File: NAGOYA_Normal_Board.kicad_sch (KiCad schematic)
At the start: 93 parts, among them CN1 value, CN10 value, CN11 value, CN12 value, CN13 value, CN14 RefereeSystem, CN15 micro_B, CN2 value, CN3 value, CN4 value, CN5 value, CN6 value, CN7 value, CN8 value, CN9 value, J1 debug, Q2 DDTC114EUA-7-F, U1 Teensy4.1, U2 TCAN1042HVDR, U3 TCAN1042HVDR, U4 TCAN1042HVDR, U5 FT234XD, U6 TLP172AM, U7 BNO055, U9 LXES11DAA2-137, Y2 32.768 k

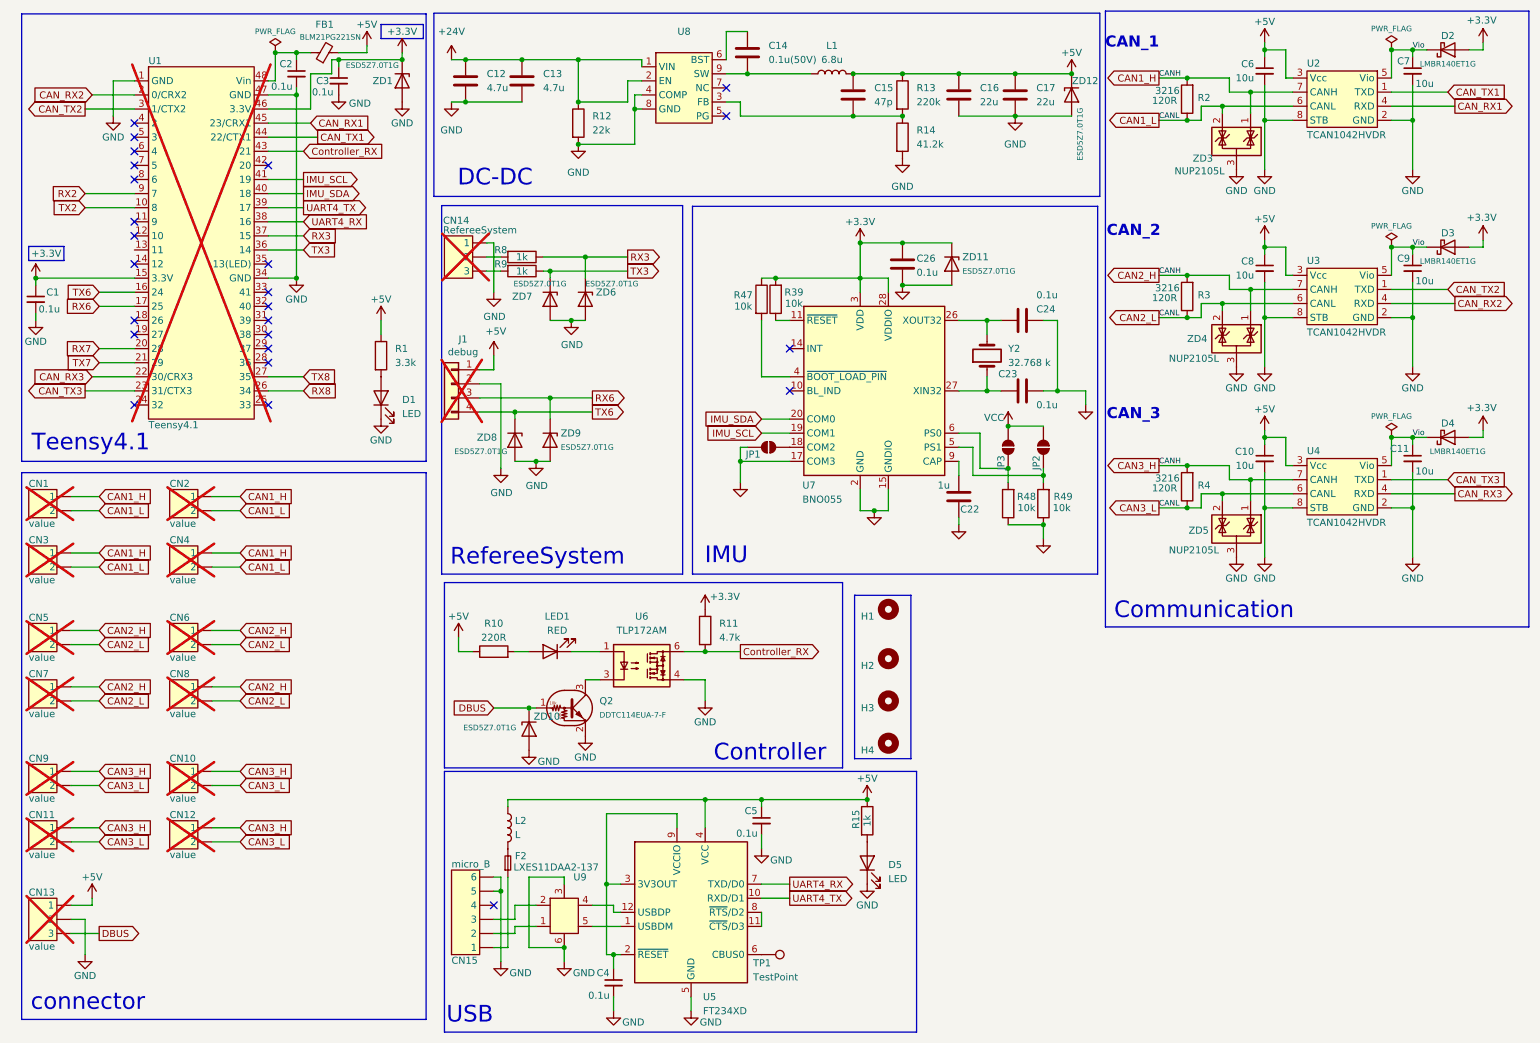
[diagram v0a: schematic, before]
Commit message: Update
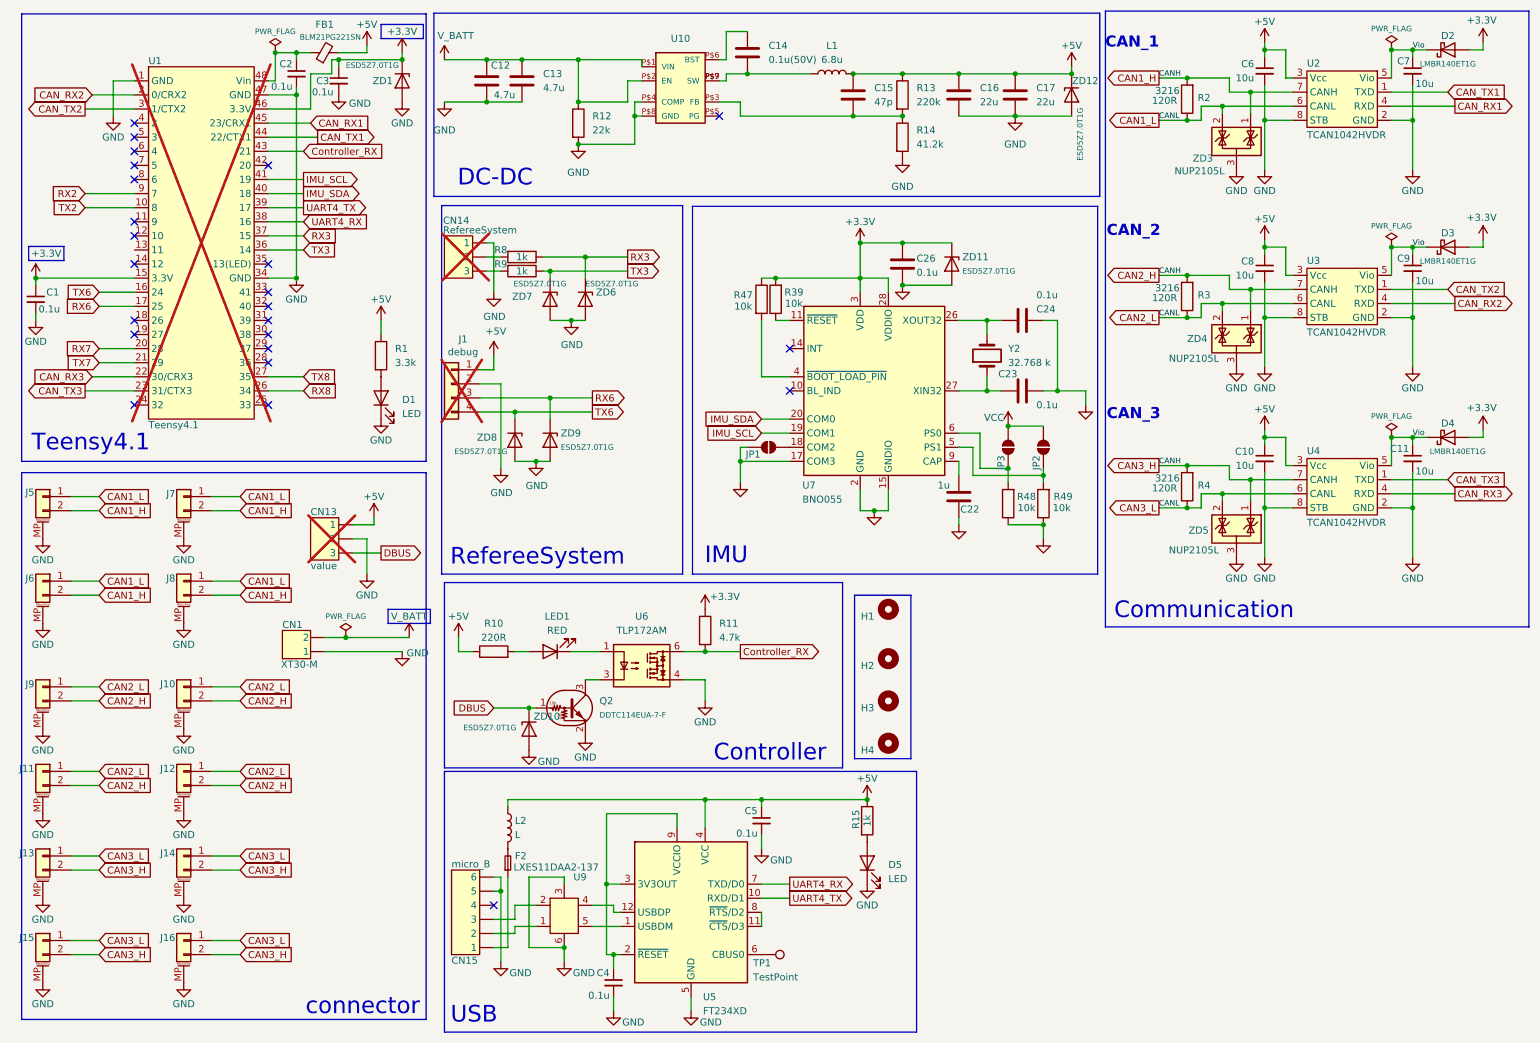
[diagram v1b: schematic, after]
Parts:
- removed CN10, CN11, CN12, CN2, CN3, CN4, CN5, CN6, CN7, CN8, CN9: value, symbol 0_circuit:CON_2P
- removed U8: ~, TanekonModule:V-DFN3020-13-A_L3.0-W2.0-P0.45-BL-EP_AP6335X, symbol TanekonModule:AP63357DV-7
- added J10, J11, J12, J13, J14, J15, J16, J5, J6, J7, J8, J9: CAN3, Connector_JST:JST_GH_SM02B-GHS-TB_1x02-1MP_P1.25mm_Horizontal, symbol Connector_Generic_MountingPin:Conn_01x02_MountingPin
- added U10: AP63357, 0_PCB:V-DFN3020-13, symbol AP63357:AP63357
- CN1: value value -> XT30-M; footprint (none) -> 0_PCB:AMASS_XT30PW-M_1x02_P2.50mm_Horizontal; LCSC (none) -> C428721; 型番 (none) -> XT30PW-M30.G.Y; 購入先 (none) -> JLCPCB; 購入先URL (none) -> https://jlcpcb.com/partdetail/Changzhou_AmassElec-XT30UM/C9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; now fitted
- CN13: footprint (none) -> Connector_PinHeader_2.54mm:PinHeader_1x03_P2.54mm_Vertical
- CN14: footprint (none) -> Connector_JST:JST_XH_B3B-XH-AM_1x03_P2.50mm_Vertical
- CN15: footprint (none) -> Connector_USB:USB_Micro-B_Amphenol_10118194-0001LF_Horizontal
- F2: footprint (none) -> Fuse:Fuse_0603_1608Metric; LCSC (none) -> C116602
- L2: footprint (none) -> Inductor_SMD:L_0603_1608Metric; LCSC (none) -> C85834
- U9: footprint (none) -> 0_PCB:FIL_LXES11DAA2-137
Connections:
- net CAN1_H: now also J10.2 (Pin_2), J11.2 (Pin_2), J12.2 (Pin_2), J13.2 (Pin_2), J14.2 (Pin_2), J15.2 (Pin_2), J16.2 (Pin_2), J5.2 (Pin_2), J6.2 (Pin_2), J7.2 (Pin_2), J8.2 (Pin_2), J9.2 (Pin_2); no longer CN1.1
- net CAN1_L: now also J10.1 (Pin_1), J11.1 (Pin_1), J12.1 (Pin_1), J13.1 (Pin_1), J14.1 (Pin_1), J15.1 (Pin_1), J16.1 (Pin_1), J5.1 (Pin_1), J6.1 (Pin_1), J7.1 (Pin_1), J8.1 (Pin_1), J9.1 (Pin_1); no longer CN1.2
- net GND: now also CN1.1, J10.MP (MountPin), J11.MP (MountPin), J12.MP (MountPin), J13.MP (MountPin), J14.MP (MountPin), J15.MP (MountPin), J16.MP (MountPin), J5.MP (MountPin), J6.MP (MountPin), J7.MP (MountPin), J8.MP (MountPin), J9.MP (MountPin), U10.P$4 (COMP), U10.P$8 (GND)
- net at C14.1: now also U10.P$6 (BST)
- net at C14.2, L1.1: now also U10.P$7 (SW), U10.P$9 (SW)
- net at C15.2, R13.2, R14.1: now also U10.P$3 (FB)
- net +24V renamed V_BATT
- net V_BATT: now also CN1.2, U10.P$1 (VIN), U10.P$2 (EN)
- no-connect marks 25 -> 24
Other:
- moved on the sheet: C12, CN13
